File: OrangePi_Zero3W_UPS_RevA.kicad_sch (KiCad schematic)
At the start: 6 parts, among them J1 ORANGE_PI_ZERO_3W_HEADER, J2 BATTERY_1S_PROTECTED_NTC, U1 MAX17048G_T10

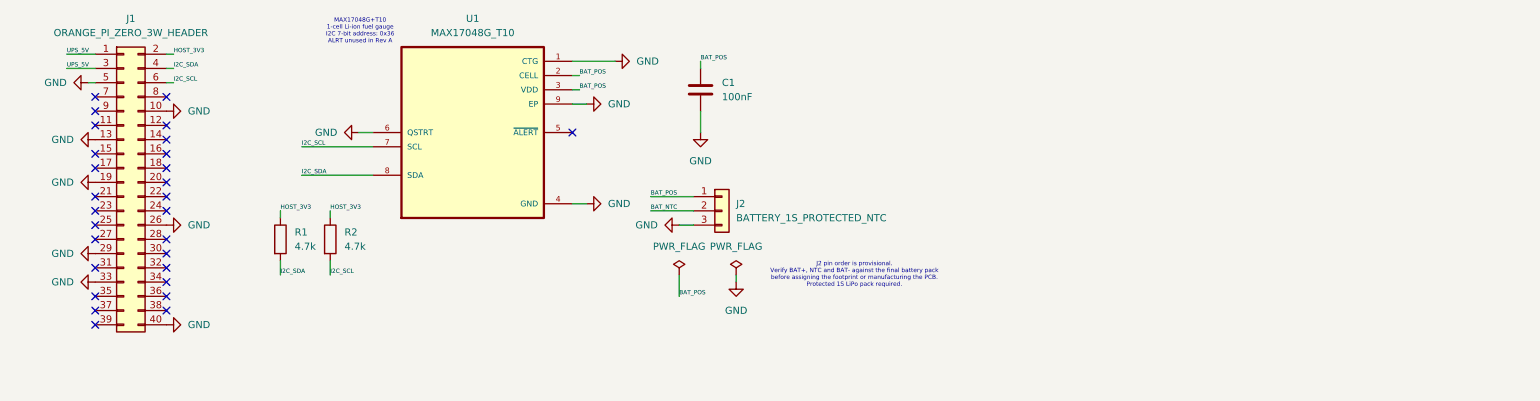
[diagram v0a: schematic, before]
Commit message: phase 5B.1B
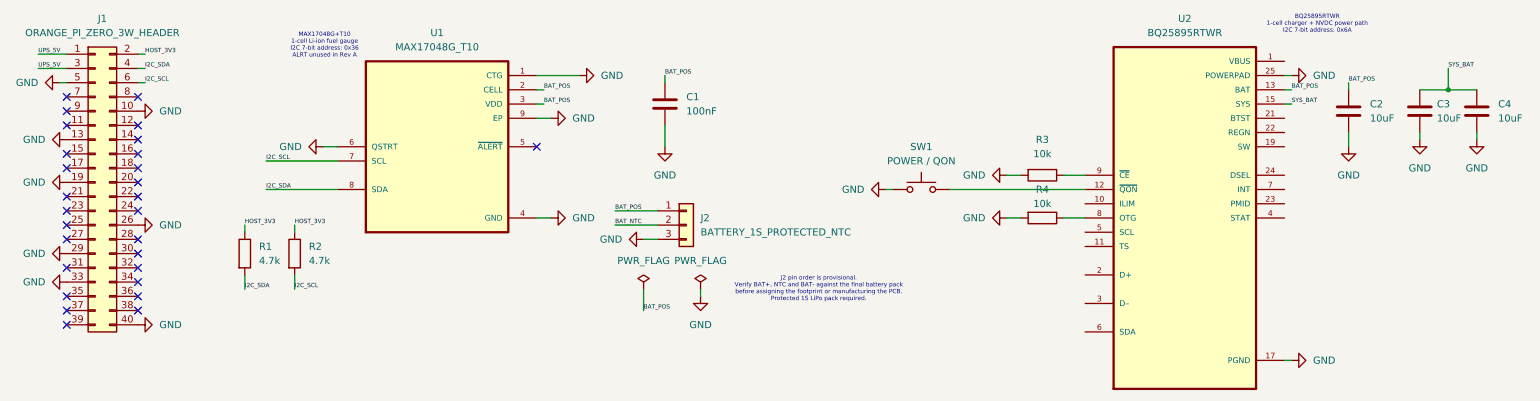
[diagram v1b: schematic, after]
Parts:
- added C2, C3, C4: 10uF, Capacitor_SMD:C_0805_2012Metric, symbol Device:C
- added R3, R4: 10k, Resistor_SMD:R_0603_1608Metric, symbol Device:R
- added SW1: POWER / QON, symbol Switch:SW_Push
- added U2: BQ25895RTWR, BQ25895RTWR:QFN50P400X400X80-25N, symbol BQ25895RTWR:BQ25895RTWR
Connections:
- net GND: now also C2.2, C3.2, C4.2, R3.2, R4.2, SW1.1, U2.17 (PGND), U2.18 (PGND), U2.25 (POWERPAD)
- net BAT_POS renamed BAT
- net BAT: now also C2.1, U2.13 (BAT), U2.14 (BAT)
- new net: SW1.2, U2.12 (~{QON})
- new net: R4.1, U2.8 (OTG)
- new net: R3.1, U2.9 (~{CE})
- new net SW: U2.19 (SW), U2.20 (SW)
- new net SYS: C3.1, C4.1, U2.15 (SYS), U2.16 (SYS)
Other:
- note added: "BQ25895RTWR 1-cell charger + NVDC power path I2C 7-bit address: 0x6A"
- moved on the sheet: C1, J1, J2, R1, R2, U1
